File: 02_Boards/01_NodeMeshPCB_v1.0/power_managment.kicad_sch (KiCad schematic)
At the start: 0 parts

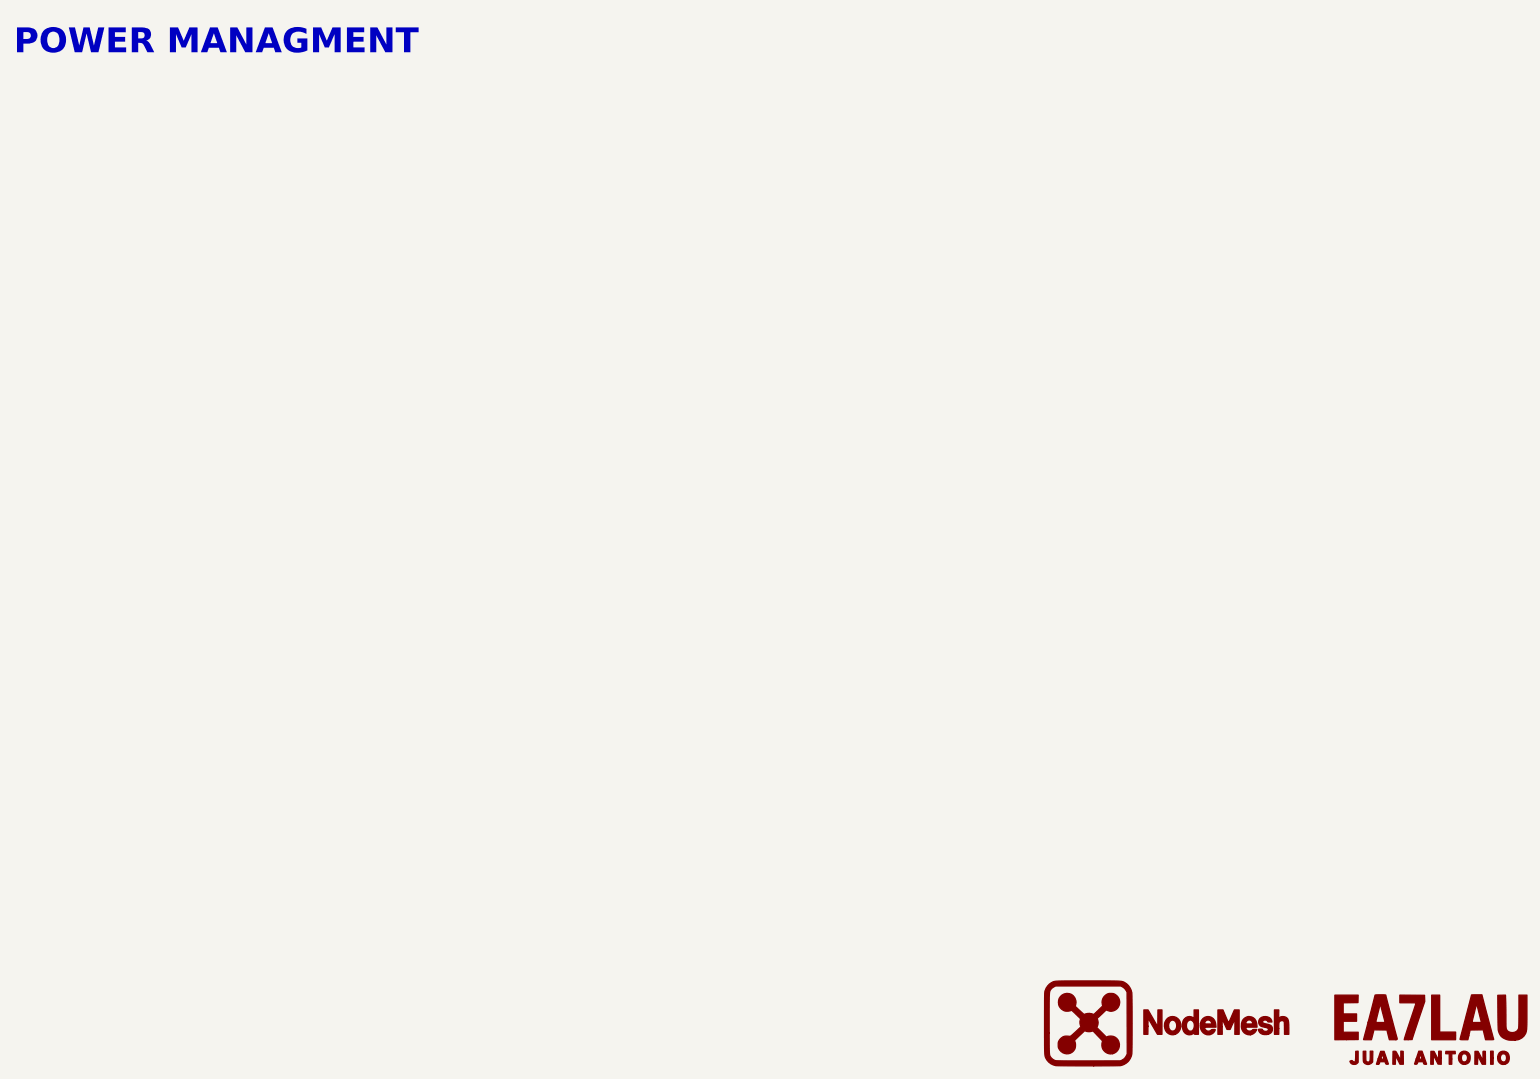
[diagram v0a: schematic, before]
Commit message: mppt solar charger schematic
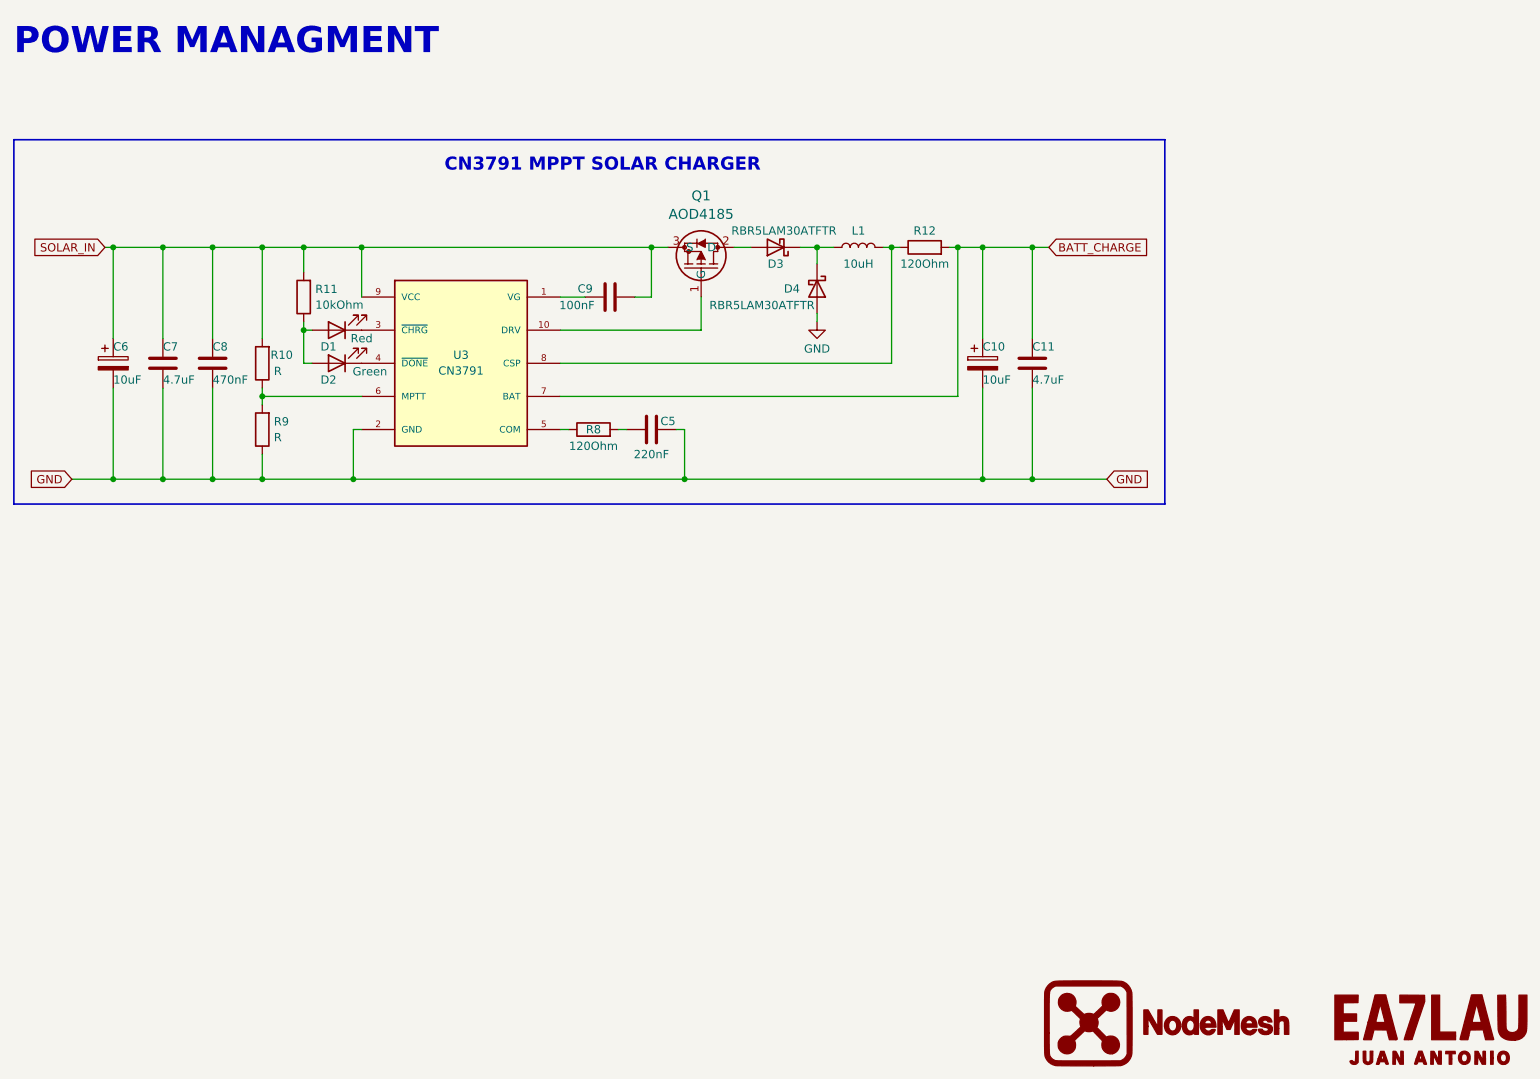
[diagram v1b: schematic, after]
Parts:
- added C10, C6: 10uF, symbol Device:C_Polarized
- added C11, C7: 4.7uF, symbol Device:C
- added C5: 220nF, symbol Device:C
- added C8: 470nF, symbol Device:C
- added C9: 100nF, symbol Device:C
- added D1: Red, symbol Device:LED
- added D2: Green, symbol Device:LED
- added D3, D4: RBR5LAM30ATFTR, symbol Device:D_Schottky
- added L1: 10uH, symbol Device:L
- added Q1: AOD4185, TO252_AOS, symbol AOD4185:AOD4185
- added R10, R9: R, symbol Device:R
- added R11: 10kOhm, symbol Device:R
- added R12, R8: 120Ohm, symbol Device:R
- added U3: CN3791, CN3791:SSOP-10-1MM, symbol CN3791:CN3791
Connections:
- new net: Q1.1 (G), U3.10 (DRV)
- new net: D3.2 (A), Q1.2 (D)
- new net: R8.1, U3.5 (COM)
- new net: C5.1, R8.2
- new net: D3.1 (K), D4.1 (K), L1.1
- new net: C9.1, U3.1 (VG)
- new net: D1.1 (K), U3.3 (~{CHRG})
- new net: D2.1 (K), U3.4 (~{DONE})
- new net: R10.1, R9.2, U3.6 (MPTT)
- new net: L1.2, R12.1, U3.8 (CSP)
- new net: D1.2 (A), D2.2 (A), R11.1
- new net BATT_CHARGE: C10.1, C11.1, R12.2, U3.7 (BAT)
- new net GND: C10.2, C11.2, C5.2, C6.2, C7.2, C8.2, D4.2 (A), R9.1, U3.2 (GND)
- new net SOLAR_IN: C6.1, C7.1, C8.1, C9.2, Q1.3 (S), R10.2, R11.2, U3.9 (VCC)
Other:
- note added: "CN3791 MPPT SOLAR CHARGER"
